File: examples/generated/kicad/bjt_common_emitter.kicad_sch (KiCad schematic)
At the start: 6 parts, among them Q1 2N3904

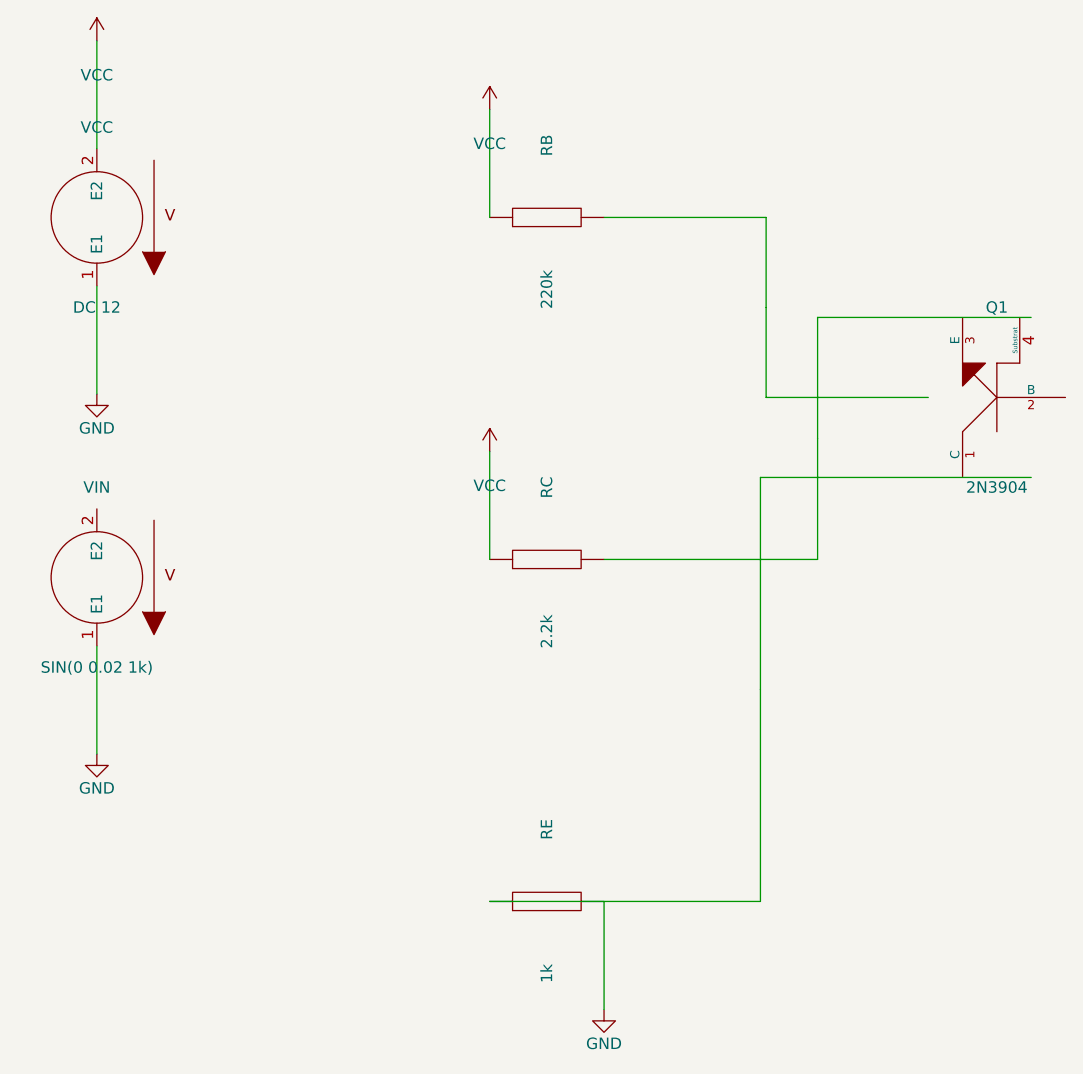
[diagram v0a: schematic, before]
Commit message: Attempt to correct strange wiring.
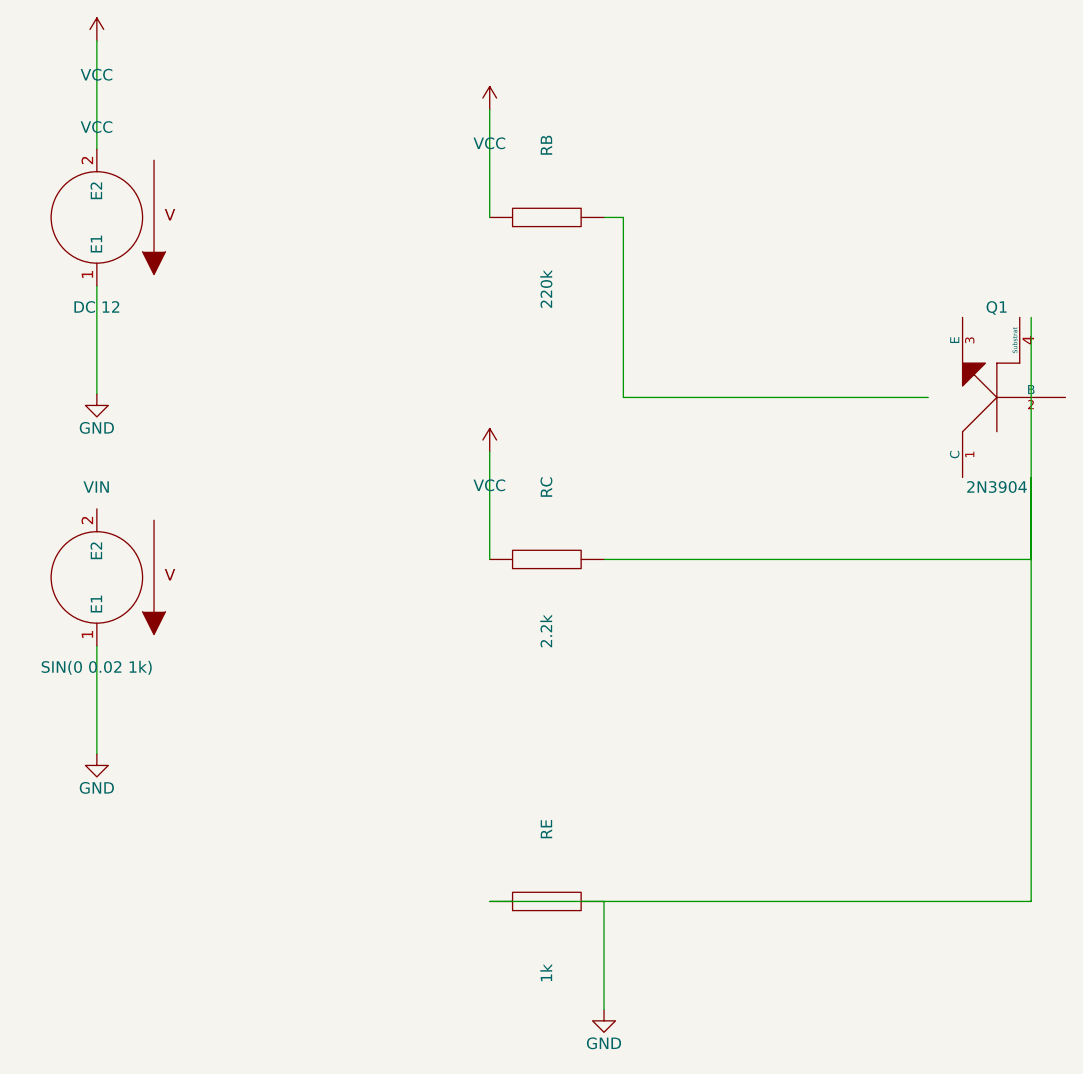
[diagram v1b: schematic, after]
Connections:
- net at RE.1: now also RC.2
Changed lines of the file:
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@@
     (stroke (width 0) (type solid) (color 0 0 0 0))
   )
-  (wire (pts (xy 106.35 70.00) (xy 124.36 70.00))
+  (wire (pts (xy 106.35 70.00) (xy 108.50 70.00))
     (stroke (width 0) (type solid) (color 0 0 0 0))
   )
-  (wire (pts (xy 124.36 70.00) (xy 124.36 80.00))
+  (wire (pts (xy 108.50 70.00) (xy 108.50 90.00))
     (stroke (width 0) (type solid) (color 0 0 0 0))
   )
-  (wire (pts (xy 142.38 90.00) (xy 124.36 90.00))
+  (wire (pts (xy 108.50 90.00) (xy 142.38 90.00))
     (stroke (width 0) (type solid) (color 0 0 0 0))
   )
-  (wire (pts (xy 124.36 90.00) (xy 124.36 80.00))
+  (wire (pts (xy 106.35 108.00) (xy 153.81 108.00))
     (stroke (width 0) (type solid) (color 0 0 0 0))
   )
-  (wire (pts (xy 106.35 108.00) (xy 130.08 108.00))
+  (wire (pts (xy 153.81 108.00) (xy 153.81 81.11))
     (stroke (width 0) (type solid) (color 0 0 0 0))
   )
-  (wire (pts (xy 130.08 108.00) (xy 130.08 94.56))
+  (wire (pts (xy 93.65 146.00) (xy 153.81 146.00))
     (stroke (width 0) (type solid) (color 0 0 0 0))
   )
-  (wire (pts (xy 153.81 81.11) (xy 130.08 81.11))
+  (wire (pts (xy 153.81 146.00) (xy 153.81 98.89))
     (stroke (width 0) (type solid) (color 0 0 0 0))
   )
-  (wire (pts (xy 130.08 81.11) (xy 130.08 94.56))
-    (stroke (width 0) (type solid) (color 0 0 0 0))
-  )
-  (wire (pts (xy 93.65 146.00) (xy 123.73 146.00))
-    (stroke (width 0) (type solid) (color 0 0 0 0))
-  )
-  (wire (pts (xy 123.73 146.00) (xy 123.73 122.44))
-    (stroke (width 0) (type solid) (color 0 0 0 0))
-  )
-  (wire (pts (xy 153.81 98.89) (xy 123.73 98.89))
-    (stroke (width 0) (type solid) (color 0 0 0 0))
-  )
-  (wire (pts (xy 123.73 98.89) (xy 123.73 122.44))
-    (stroke (width 0) (type solid) (color 0 0 0 0))
-  )

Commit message: Attempt shape and wiring fixes again.
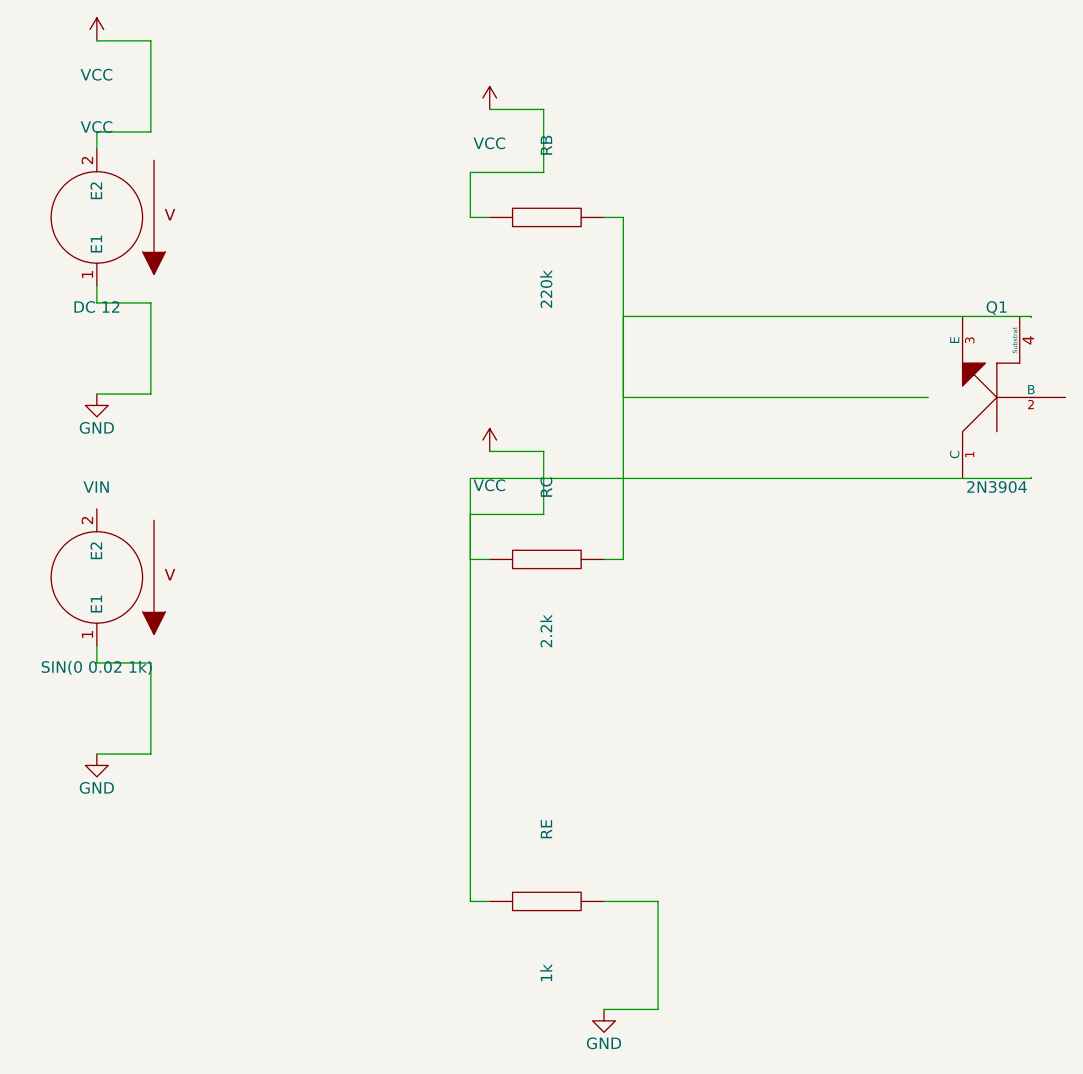
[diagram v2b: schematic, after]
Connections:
- net VCC: now also RE.1
- net at RB.2: now also RC.2
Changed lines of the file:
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@@
     )
   )
-  (wire (pts (xy 50.00 62.38) (xy 50.00 50.38))
+  (wire (pts (xy 50.00 62.38) (xy 50.00 60.50))
     (stroke (width 0) (type solid) (color 0 0 0 0))
   )
-  (wire (pts (xy 50.00 77.62) (xy 50.00 89.62))
+  (wire (pts (xy 50.00 60.50) (xy 56.00 60.50))
     (stroke (width 0) (type solid) (color 0 0 0 0))
   )
-  (wire (pts (xy 50.00 117.62) (xy 50.00 129.62))
+  (wire (pts (xy 56.00 60.50) (xy 56.00 50.38))
     (stroke (width 0) (type solid) (color 0 0 0 0))
   )
-  (wire (pts (xy 93.65 70.00) (xy 93.65 58.00))
+  (wire (pts (xy 56.00 50.38) (xy 50.00 50.38))
     (stroke (width 0) (type solid) (color 0 0 0 0))
   )
-  (wire (pts (xy 93.65 108.00) (xy 93.65 96.00))
+  (wire (pts (xy 50.00 77.62) (xy 50.00 79.50))
     (stroke (width 0) (type solid) (color 0 0 0 0))
   )
-  (wire (pts (xy 106.35 146.00) (xy 106.35 158.00))
+  (wire (pts (xy 50.00 79.50) (xy 56.00 79.50))
+    (stroke (width 0) (type solid) (color 0 0 0 0))
+  )
+  (wire (pts (xy 56.00 79.50) (xy 56.00 89.62))
+    (stroke (width 0) (type solid) (color 0 0 0 0))
+  )
+  (wire (pts (xy 56.00 89.62) (xy 50.00 89.62))
+    (stroke (width 0) (type solid) (color 0 0 0 0))
+  )
+  (wire (pts (xy 50.00 117.62) (xy 50.00 119.50))
+    (stroke (width 0) (type solid) (color 0 0 0 0))
+  )
+  (wire (pts (xy 50.00 119.50) (xy 56.00 119.50))
+    (stroke (width 0) (type solid) (color 0 0 0 0))
+  )
+  (wire (pts (xy 56.00 119.50) (xy 56.00 129.62))
+    (stroke (width 0) (type solid) (color 0 0 0 0))
+  )
+  (wire (pts (xy 56.00 129.62) (xy 50.00 129.62))
+    (stroke (width 0) (type solid) (color 0 0 0 0))
+  )
+  (wire (pts (xy 93.65 70.00) (xy 91.50 70.00))
+    (stroke (width 0) (type solid) (color 0 0 0 0))
+  )
+  (wire (pts (xy 91.50 70.00) (xy 91.50 65.00))
+    (stroke (width 0) (type solid) (color 0 0 0 0))
+  )
+  (wire (pts (xy 91.50 65.00) (xy 99.65 65.00))
+    (stroke (width 0) (type solid) (color 0 0 0 0))
+  )
+  (wire (pts (xy 99.65 65.00) (xy 99.65 58.00))
+    (stroke (width 0) (type solid) (color 0 0 0 0))
+  )
+  (wire (pts (xy 99.65 58.00) (xy 93.65 58.00))
+    (stroke (width 0) (type solid) (color 0 0 0 0))
+  )
+  (wire (pts (xy 93.65 108.00) (xy 91.50 108.00))
+    (stroke (width 0) (type solid) (color 0 0 0 0))
+  )
+  (wire (pts (xy 91.50 108.00) (xy 91.50 103.00))
+    (stroke (width 0) (type solid) (color 0 0 0 0))
+  )
+  (wire (pts (xy 91.50 103.00) (xy 99.65 103.00))
+    (stroke (width 0) (type solid) (color 0 0 0 0))
+  )
+  (wire (pts (xy 99.65 103.00) (xy 99.65 96.00))
+    (stroke (width 0) (type solid) (color 0 0 0 0))
+  )
+  (wire (pts (xy 99.65 96.00) (xy 93.65 96.00))
+    (stroke (width 0) (type solid) (color 0 0 0 0))
+  )
+  (wire (pts (xy 106.35 146.00) (xy 112.35 146.00))
+    (stroke (width 0) (type solid) (color 0 0 0 0))
+  )
+  (wire (pts (xy 112.35 146.00) (xy 112.35 158.00))
+    (stroke (width 0) (type solid) (color 0 0 0 0))
+  )
+  (wire (pts (xy 112.35 158.00) (xy 106.35 158.00))
     (stroke (width 0) (type solid) (color 0 0 0 0))
   )
@@
     (stroke (width 0) (type solid) (color 0 0 0 0))
   )
-  (wire (pts (xy 106.35 108.00) (xy 153.81 108.00))
+  (wire (pts (xy 106.35 108.00) (xy 108.50 108.00))
     (stroke (width 0) (type solid) (color 0 0 0 0))
   )
-  (wire (pts (xy 153.81 108.00) (xy 153.81 81.11))
+  (wire (pts (xy 108.50 108.00) (xy 108.50 81.00))
     (stroke (width 0) (type solid) (color 0 0 0 0))
   )
-  (wire (pts (xy 93.65 146.00) (xy 153.81 146.00))
+  (wire (pts (xy 108.50 81.00) (xy 153.81 81.00))
     (stroke (width 0) (type solid) (color 0 0 0 0))
   )
-  (wire (pts (xy 153.81 146.00) (xy 153.81 98.89))
+  (wire (pts (xy 153.81 81.00) (xy 153.81 81.11))
     (stroke (width 0) (type solid) (color 0 0 0 0))
   )
+  (wire (pts (xy 93.65 146.00) (xy 91.50 146.00))
+    (stroke (width 0) (type solid) (color 0 0 0 0))
+  )
+  (wire (pts (xy 91.50 146.00) (xy 91.50 99.00))
+    (stroke (width 0) (type solid) (color 0 0 0 0))
+  )
+  (wire (pts (xy 91.50 99.00) (xy 153.81 99.00))
+    (stroke (width 0) (type solid) (color 0 0 0 0))
+  )
+  (wire (pts (xy 153.81 99.00) (xy 153.81 98.89))
+    (stroke (width 0) (type solid) (color 0 0 0 0))
+  )
